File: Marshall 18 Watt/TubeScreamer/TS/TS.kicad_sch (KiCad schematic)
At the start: 24 parts, among them J1 Barrel_Jack_Switch, J2 BAT, J3 IN, Q1 2SC1815, U1 RC4558

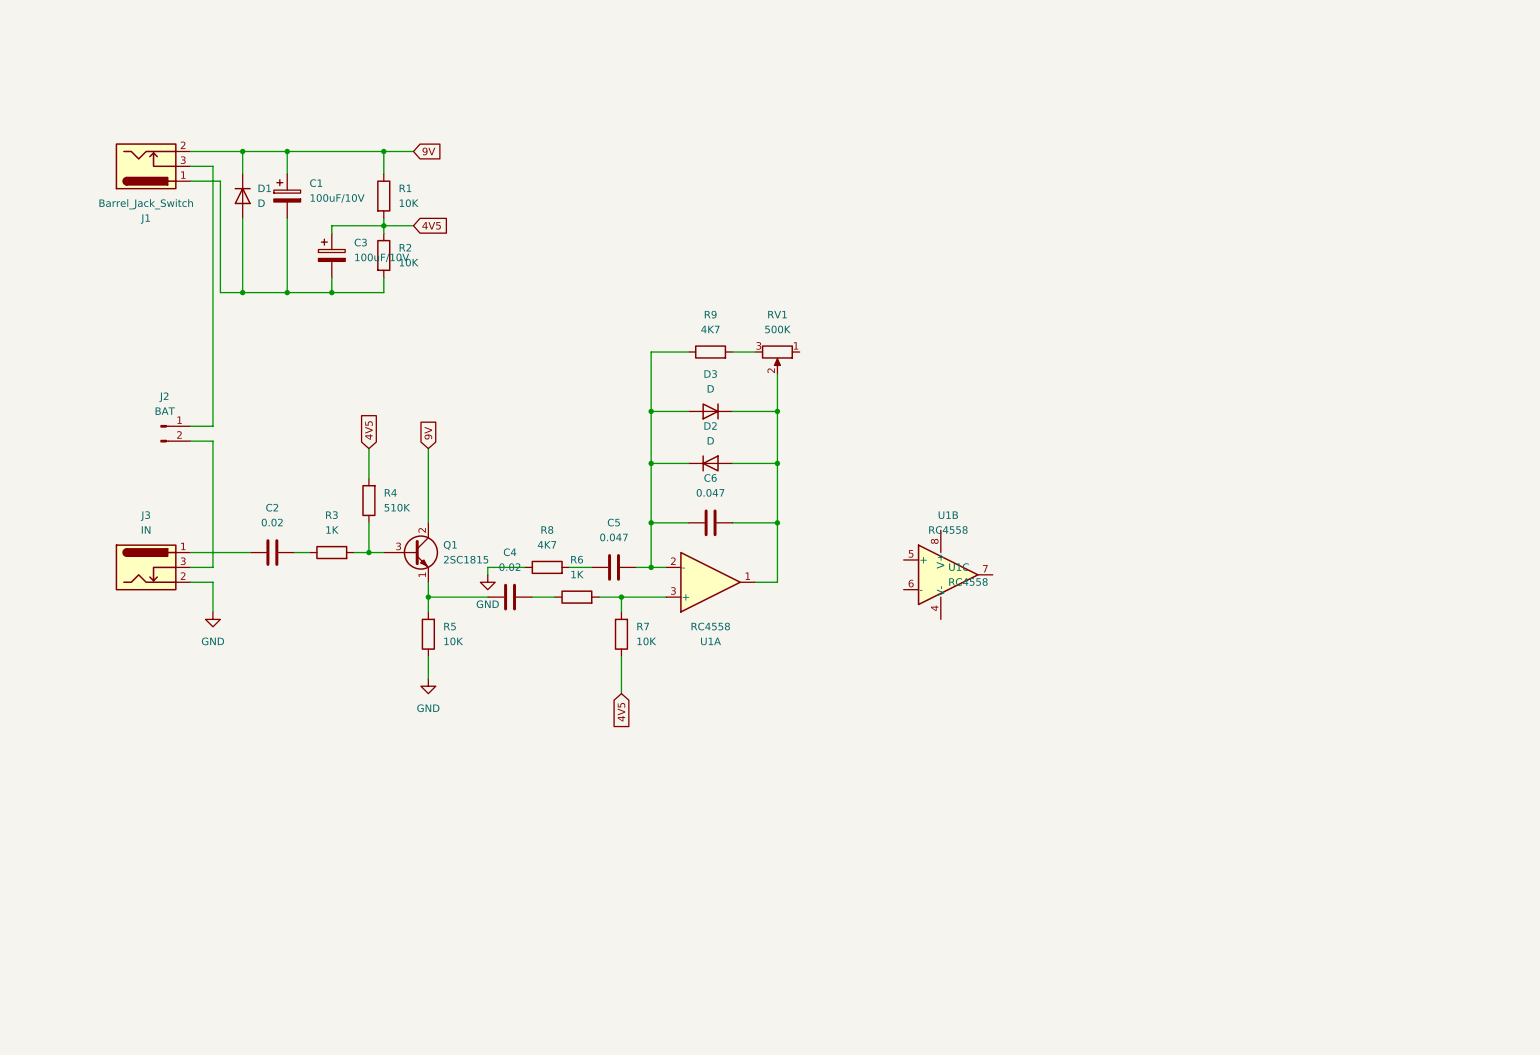
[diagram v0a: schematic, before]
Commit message: Update 27_03_25
Add TS
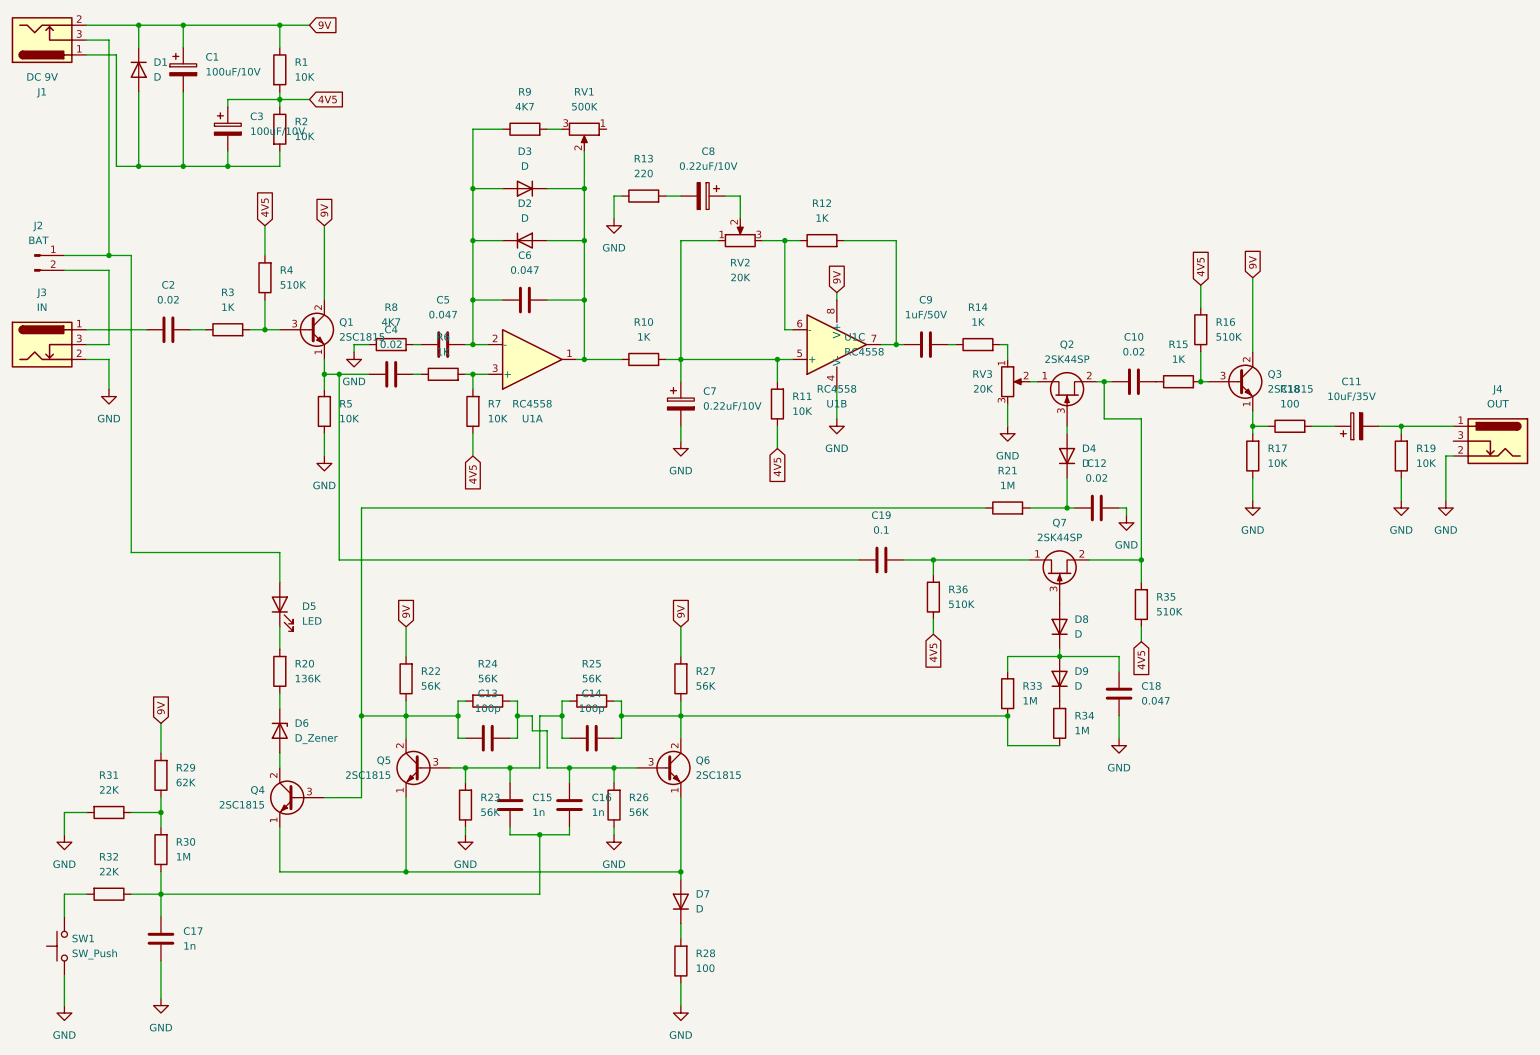
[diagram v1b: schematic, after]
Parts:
- added C10, C12: 0.02, Capacitor_THT:C_Disc_D4.3mm_W1.9mm_P5.00mm, symbol Device:C
- added C11: 10uF/35V, Capacitor_THT:CP_Radial_D5.0mm_P2.50mm, symbol Device:C_Polarized
- added C13, C14: 100p, Capacitor_THT:C_Disc_D4.3mm_W1.9mm_P5.00mm, symbol Device:C
- added C15, C16, C17: 1n, Capacitor_THT:C_Disc_D4.3mm_W1.9mm_P5.00mm, symbol Device:C
- added C18: 0.047, Capacitor_THT:C_Disc_D4.3mm_W1.9mm_P5.00mm, symbol Device:C
- added C19: 0.1, Capacitor_THT:C_Disc_D4.3mm_W1.9mm_P5.00mm, symbol Device:C
- added C7, C8: 0.22uF/10V, Capacitor_THT:CP_Radial_D5.0mm_P2.50mm, symbol Device:C_Polarized
- added C9: 1uF/50V, Capacitor_THT:C_Disc_D4.3mm_W1.9mm_P5.00mm, symbol Device:C
- added D4, D7, D8, D9: D, Diode_THT:D_A-405_P7.62mm_Horizontal, symbol Device:D
- added D5: LED, LED_THT:LED_D3.0mm, symbol Device:LED
- added D6: D_Zener, Diode_THT:D_DO-35_SOD27_P7.62mm_Horizontal, symbol Device:D_Zener
- added J4: OUT, Connector_PinHeader_2.54mm:PinHeader_1x03_P2.54mm_Vertical, symbol Connector:Barrel_Jack_Switch
- added Q2, Q7: 2SK44SP, Package_TO_SOT_THT:TO-92L_Inline, symbol Device:Q_NJFET_DSG
- added Q3, Q4, Q5, Q6: 2SC1815, Package_TO_SOT_THT:TO-92_Inline, symbol Transistor_BJT:2SC1815
- added R10, R12, R14, R15: 1K, Resistor_THT:R_Axial_DIN0207_L6.3mm_D2.5mm_P7.62mm_Horizontal, symbol Device:R
- added R11, R17, R19: 10K, Resistor_THT:R_Axial_DIN0207_L6.3mm_D2.5mm_P7.62mm_Horizontal, symbol Device:R
- added R13: 220, Resistor_THT:R_Axial_DIN0207_L6.3mm_D2.5mm_P7.62mm_Horizontal, symbol Device:R
- added R16, R35, R36: 510K, Resistor_THT:R_Axial_DIN0207_L6.3mm_D2.5mm_P7.62mm_Horizontal, symbol Device:R
- added R18, R28: 100, Resistor_THT:R_Axial_DIN0207_L6.3mm_D2.5mm_P7.62mm_Horizontal, symbol Device:R
- added R20: 136K, Resistor_THT:R_Axial_DIN0207_L6.3mm_D2.5mm_P7.62mm_Horizontal, symbol Device:R
- added R21, R30, R33, R34: 1M, Resistor_THT:R_Axial_DIN0207_L6.3mm_D2.5mm_P7.62mm_Horizontal, symbol Device:R
- added R22, R23, R24, R25, R26, R27: 56K, Resistor_THT:R_Axial_DIN0207_L6.3mm_D2.5mm_P7.62mm_Horizontal, symbol Device:R
- added R29: 62K, Resistor_THT:R_Axial_DIN0207_L6.3mm_D2.5mm_P7.62mm_Horizontal, symbol Device:R
- added R31, R32: 22K, Resistor_THT:R_Axial_DIN0207_L6.3mm_D2.5mm_P7.62mm_Horizontal, symbol Device:R
- added RV2, RV3: 20K, Potentiometer_THT:Potentiometer_Omeg_PC16BU_Vertical, symbol Device:R_Potentiometer
- added SW1: SW_Push, Connector_PinHeader_2.54mm:PinHeader_1x02_P2.54mm_Vertical, symbol Switch:SW_Push
- J1: value Barrel_Jack_Switch -> DC 9V
- J2: footprint (none) -> Connector_PinHeader_2.54mm:PinHeader_1x02_P2.54mm_Vertical
- J3: footprint (none) -> Connector_PinHeader_2.54mm:PinHeader_1x03_P2.54mm_Vertical
- RV1: footprint (none) -> Potentiometer_THT:Potentiometer_Omeg_PC16BU_Vertical
- U1: footprint (none) -> Package_DIP:DIP-8_W7.62mm_Socket
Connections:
- net 4V5: now also R11.1, R16.2, R35.1, R36.1
- net 9V: now also U1.8 (V+), Q3.2 (C), R22.2, R27.2, R29.2
- net GND: now also U1.4 (V-), C12.2, C17.1, C18.1, C7.2, J4.2, R13.1, R17.1, R19.1, R23.1, R26.1, R28.1, R31.2, RV3.3, SW1.1
- net at J1.3, J2.1 (Pin_1): now also D5.2 (A)
- net at C4.1, Q1.1 (E), R5.2: now also C19.1
- net at C6.2, D2.2 (A), D3.1 (K)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: now also R10.1
- net at U1.5 (+): now also C7.1, R10.2, R11.2, RV2.1
- net at U1.6 (-): now also R12.1, RV2.3
- net at U1.7: now also C9.1, R12.2
- new net: C19.2, Q7.1 (D), R36.2
- new net: C14.2, Q6.2 (C), R25.1, R27.1, R33.1, R34.1
- new net: D9.1 (K), R34.2
- new net: D6.1 (K), R20.1
- new net: D5.1 (K), R20.2
- new net: C15.1, C16.1, C17.2, R30.1, R32.1
- new net: C13.2, C16.2, Q6.3 (B), R24.1, R26.2
- new net: Q3.1 (E), R17.2, R18.1
- new net: C11.1, R18.2
- new net: R29.1, R30.2, R31.1
- new net: Q2.1 (D), RV3.2
- new net: C10.1, Q2.2 (S), Q7.2 (S), R35.2
- new net: D4.2 (A), Q2.3 (G)
- new net: C8.1, RV2.2
- new net: C8.2, R13.2
- new net: D7.2 (A), Q4.1 (E), Q5.1 (E), Q6.1 (E)
- new net: D6.2 (A), Q4.2 (C)
- new net: C13.1, Q4.3 (B), Q5.2 (C), R21.1, R22.1, R24.2
- new net: C9.2, R14.1
- new net: C18.2, D8.1 (K), D9.2 (A), R33.2
- new net: C12.1, D4.1 (K), R21.2
- new net: R32.2, SW1.2
- new net: C11.2, J4.1, R19.2
- new net: Q3.3 (B), R15.2, R16.1
- new net: C14.1, C15.2, Q5.3 (B), R23.2, R25.2
- new net: C10.2, R15.1
- new net: R14.2, RV3.1
- new net: D7.1 (K), R28.2
- new net: D8.2 (A), Q7.3 (G)
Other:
- moved on the sheet: C1, C2, C3, C4, C5, C6, D1, D2, D3, J1, J2, J3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
